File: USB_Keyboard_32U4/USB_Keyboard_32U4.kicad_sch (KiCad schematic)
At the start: 13 parts, among them J1 USB_C_Receptacle_USB2.0_16P, J2 Conn_02x03_Odd_Even, U1 ATmega32U4-A, Y1 16mhz

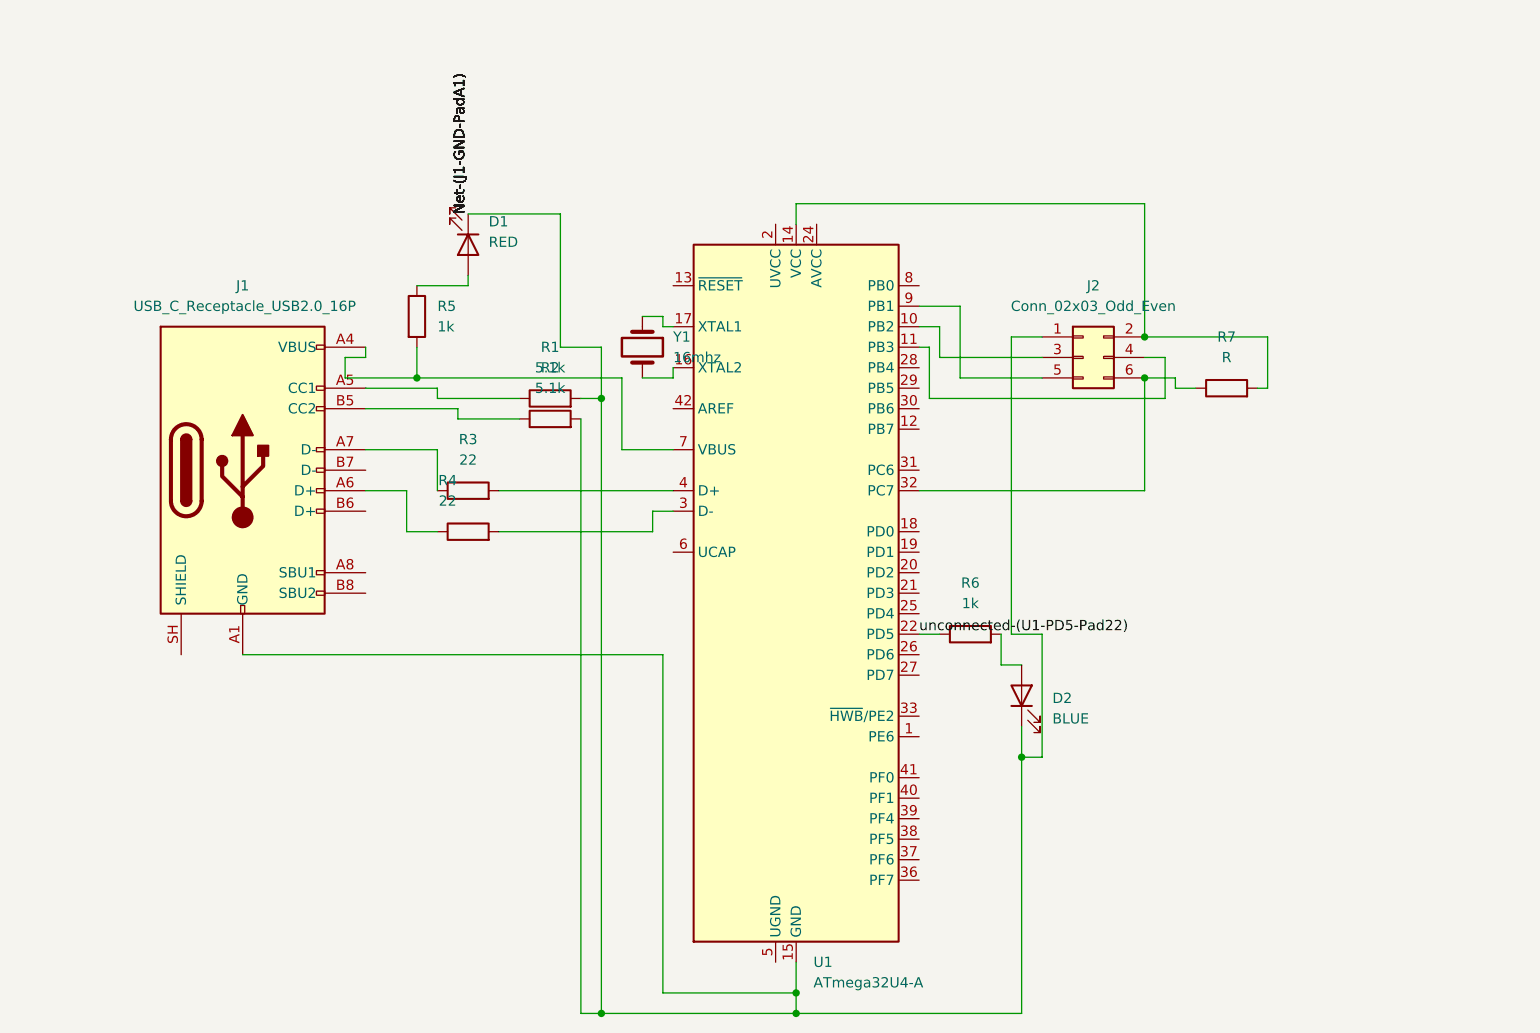
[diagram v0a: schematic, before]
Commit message: Updated schematic, pcb and bom.
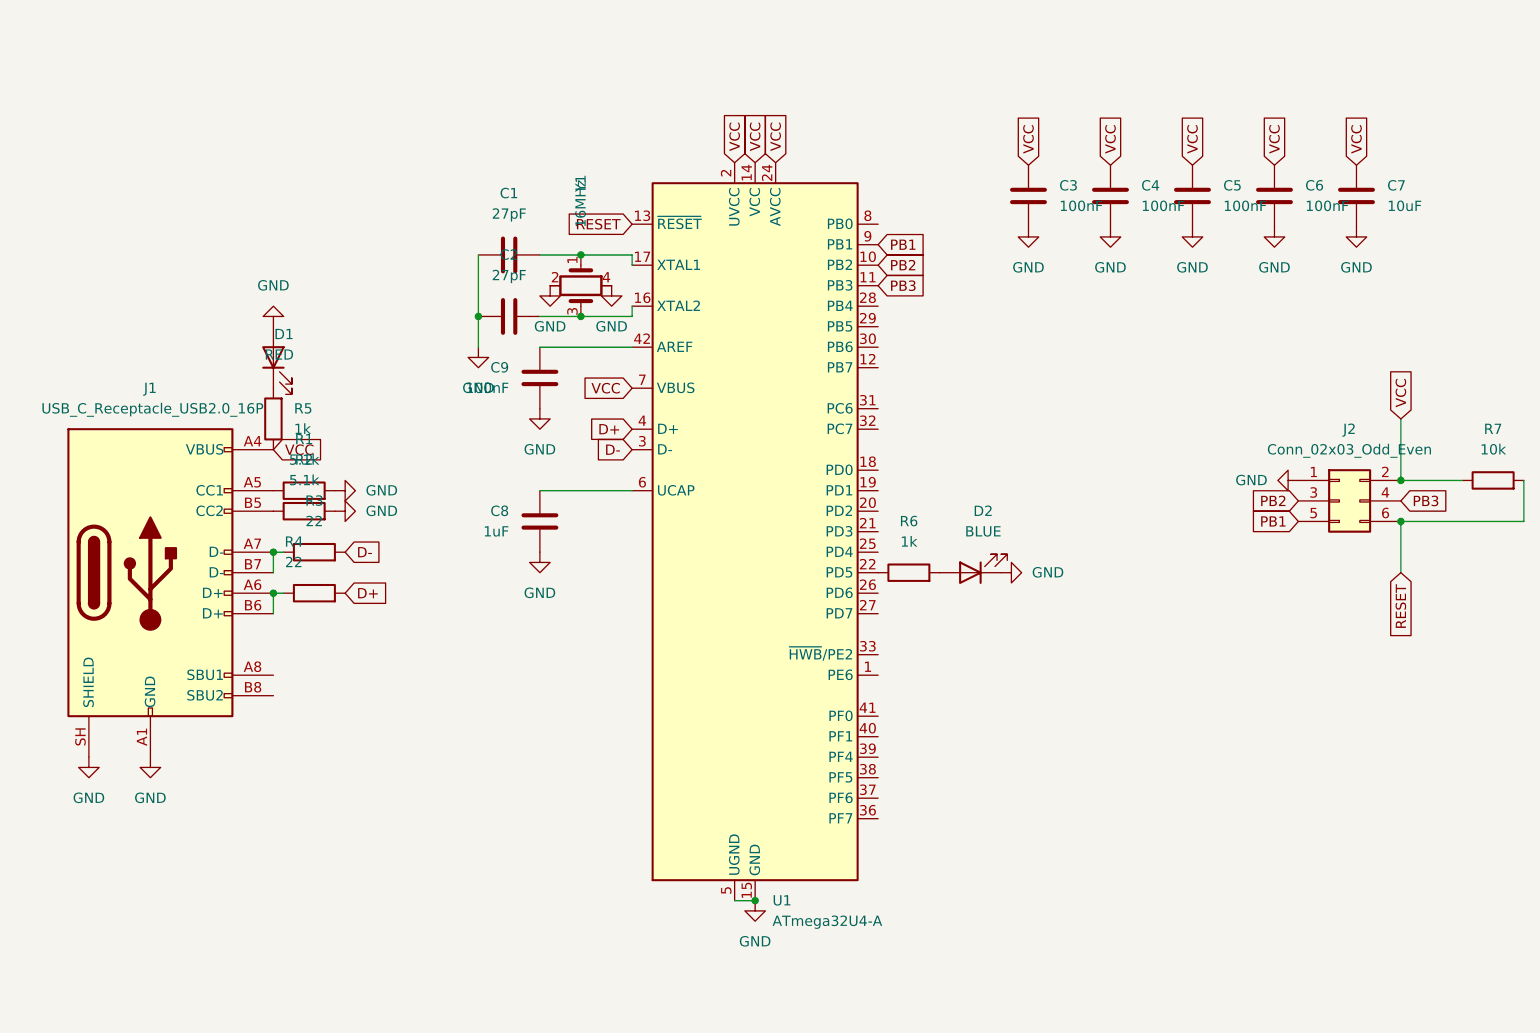
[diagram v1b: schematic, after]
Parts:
- removed Y1: 16mhz, Crystal:Crystal_SMD_3225-4Pin_3.2x2.5mm, symbol Device:Crystal
- added C1, C2: 27pF, Capacitor_SMD:C_0603_1608Metric_Pad1.08x0.95mm_HandSolder, symbol Device:C
- added C3, C4, C5, C6, C9: 100nF, Capacitor_SMD:C_0603_1608Metric_Pad1.08x0.95mm_HandSolder, symbol Device:C
- added C7: 10uF, Capacitor_SMD:C_0603_1608Metric_Pad1.08x0.95mm_HandSolder, symbol Device:C
- added C8: 1uF, Capacitor_SMD:C_0603_1608Metric_Pad1.08x0.95mm_HandSolder, symbol Device:C
- added Y1: 16MHz, Crystal:Crystal_SMD_3225-4Pin_3.2x2.5mm, symbol Device:Crystal_GND24
- D1, D2: footprint LED_SMD:LED_0805_2012Metric_Pad1.15x1.40mm_HandSolder -> LED_SMD:LED_0603_1608Metric_Pad1.05x0.95mm_HandSolder
- J2: footprint Connector_PinHeader_2.54mm:PinHeader_2x03_P2.54mm_Vertical -> 2x3 Pads:MicroKey_AVR_ISP_2x3_SMD
- R1, R2, R3, R4, R5, R6: footprint Resistor_SMD:R_0805_2012Metric_Pad1.20x1.40mm_HandSolder -> Resistor_SMD:R_0603_1608Metric_Pad0.98x0.95mm_HandSolder
- R7: value R -> 10k; footprint Resistor_SMD:R_0805_2012Metric_Pad1.20x1.40mm_HandSolder -> Resistor_SMD:R_0603_1608Metric_Pad0.98x0.95mm_HandSolder
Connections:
- net VCC: now reaches J2.2 (Pin_2), U1.14 (VCC), U1.34 (VCC)
- net VCC: now also J1.A4 (VBUS), J1.A9 (VBUS), J1.B4 (VBUS), J1.B9 (VBUS), R5.1, R7.1, U1.2 (UVCC), U1.24 (AVCC), U1.44 (AVCC), U1.7 (VBUS), C3.1, C4.1, C5.1, C6.1, C7.1; no longer R7.2
- net at J1.A6 (D+), R4.1: now also J1.B6 (D+)
- net at J1.A7 (D-), R3.1: now also J1.B7 (D-)
- net GND: now reaches J1.SH (SHIELD)
- net GND: now also D1.2 (A), D2.1 (K), J1.A1 (GND), J1.A12 (GND), J1.B1 (GND), J1.B12 (GND), J2.1 (Pin_1), R1.2, R2.2, U1.15 (GND), U1.23 (GND), U1.35 (GND), U1.43 (GND), U1.5 (UGND), C1.1, C2.1, C3.2, C4.2, C5.2, C6.2, C7.2, C8.2, C9.2, Y1.2, Y1.4
- net D+: now reaches U1.4 (D+)
- net D+: now also R4.2; no longer R3.2
- net at U1.17 (XTAL1): now also C1.2, Y1.1
- net at U1.16 (XTAL2): now also C2.2, Y1.3
- net PB2: now reaches J2.3 (Pin_3), U1.10 (PB2)
- net PB3: now reaches J2.4 (Pin_4), U1.11 (PB3)
- net RESET: now reaches U1.13 (~{RESET})
- net RESET: now also J2.6 (Pin_6), R7.2
- net D-: now reaches U1.3 (D-)
- net D-: now also R3.2; no longer R4.2
- net at U1.42 (AREF): now also C9.1
- net at U1.6 (UCAP): now also C8.1
- net PB1: now reaches J2.5 (Pin_5), U1.9 (PB1)
- removed net Net-(J1-GND-PadA1): D1.1 (K), D2.1 (K), J1.A1 (GND), J1.A12 (GND), J1.B1 (GND), J1.B12 (GND), J2.1 (Pin_1), R1.2, R2.2, U1.15 (GND), U1.23 (GND), U1.35 (GND), U1.43 (GND)
- net unconnected-(U1-PD5-Pad22): no longer names the net of R6.1, U1.22 (PD5)
- new net: D1.1 (K), R5.2
- now unconnected: U1.32 (PC7)
